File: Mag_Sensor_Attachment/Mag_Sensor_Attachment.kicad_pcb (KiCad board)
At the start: 2 copper layers, 14 x 15.8 mm, 5 parts, among them J2 Conn_01x06_Socket, U1 MA730

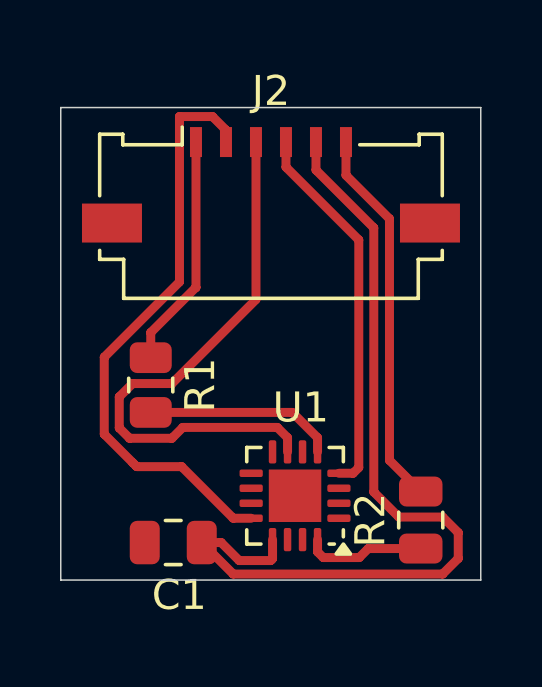
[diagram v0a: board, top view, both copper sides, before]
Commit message: Check up
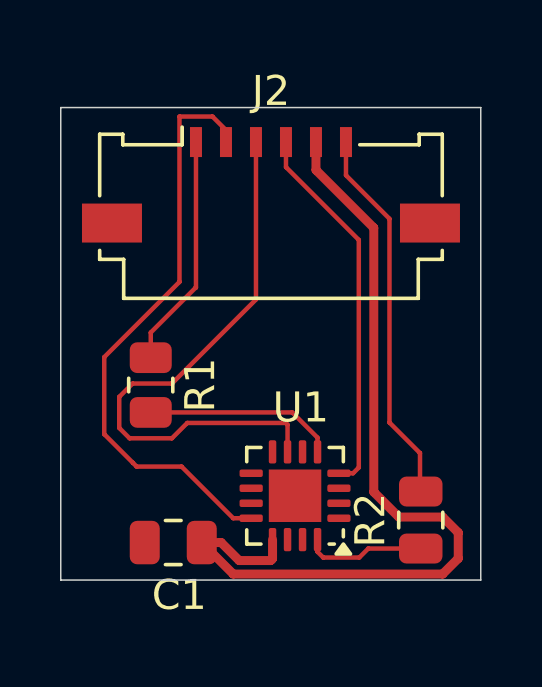
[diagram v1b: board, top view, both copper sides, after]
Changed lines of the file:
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@@
 		(start 152.434772 89.412272)
 		(end 150.0075 86.985)
-		(width 0.3)
+		(width 0.15)
 		(layer "F.Cu")
 		(net 3)
@@
 		(start 152.244772 97.19)
 		(end 152.434772 97)
-		(width 0.3)
+		(width 0.15)
 		(layer "F.Cu")
 		(net 3)
@@
 		(start 150.0075 86.985)
 		(end 150.0075 86.15)
-		(width 0.3)
+		(width 0.15)
 		(layer "F.Cu")
 		(net 3)
@@
 		(start 151.7725 97.19)
 		(end 152.244772 97.19)
-		(width 0.3)
+		(width 0.15)
 		(layer "F.Cu")
 		(net 3)
@@
 		(start 152.434772 97)
 		(end 152.434772 89.412272)
-		(width 0.3)
-		(layer "F.Cu")
-		(net 3)
-	)
-	(segment
-		(start 146.567956 95.6625)
+		(width 0.15)
+		(layer "F.Cu")
+		(net 3)
+	)
+	(segment
+		(start 144.894544 94.2)
+		(end 146.205456 94.2)
+		(width 0.15)
+		(layer "F.Cu")
+		(net 4)
+	)
+	(segment
+		(start 146.205456 96.025)
+		(end 144.794544 96.025)
+		(width 0.15)
+		(layer "F.Cu")
+		(net 4)
+	)
+	(segment
+		(start 150.06 96.4775)
+		(end 150.06 95.5725)
+		(width 0.15)
+		(layer "F.Cu")
+		(net 4)
+	)
+	(segment
+		(start 146.717956 95.5125)
 		(end 146.205456 96.025)
-		(width 0.3)
+		(width 0.15)
+		(layer "F.Cu")
+		(net 4)
+	)
+	(segment
+		(start 144.794544 96.025)
+		(end 144.45 95.680456)
+		(width 0.15)
 		(layer "F.Cu")
 		(net 4)
@@
 		(start 144.45 95.680456)
 		(end 144.45 94.644544)
-		(width 0.3)
-		(layer "F.Cu")
-		(net 4)
-	)
-	(segment
-		(start 146.205456 96.025)
-		(end 144.794544 96.025)
-		(width 0.3)
-		(layer "F.Cu")
-		(net 4)
-	)
-	(segment
-		(start 144.894544 94.2)
-		(end 146.205456 94.2)
-		(width 0.3)
+		(width 0.15)
+		(layer "F.Cu")
+		(net 4)
+	)
+	(segment
+		(start 150 95.5125)
+		(end 146.717956 95.5125)
+		(width 0.15)
+		(layer "F.Cu")
+		(net 4)
+	)
+	(segment
+		(start 149.0075 91.397956)
+		(end 149.0075 86.15)
+		(width 0.15)
+		(layer "F.Cu")
+		(net 4)
+	)
+	(segment
+		(start 144.45 94.644544)
+		(end 144.894544 94.2)
+		(width 0.15)
 		(layer "F.Cu")
 		(net 4)
@@
 		(start 146.205456 94.2)
 		(end 149.0075 91.397956)
-		(width 0.3)
-		(layer "F.Cu")
-		(net 4)
-	)
-	(segment
-		(start 149.717596 95.6625)
-		(end 146.567956 95.6625)
-		(width 0.3)
-		(layer "F.Cu")
-		(net 4)
-	)
-	(segment
-		(start 144.794544 96.025)
-		(end 144.45 95.680456)
-		(width 0.3)
-		(layer "F.Cu")
-		(net 4)
-	)
-	(segment
-		(start 149.0075 91.397956)
-		(end 149.0075 86.15)
-		(width 0.3)
-		(layer "F.Cu")
-		(net 4)
-	)
-	(segment
-		(start 150.06 96.4775)
-		(end 150.06 96.004904)
-		(width 0.3)
-		(layer "F.Cu")
-		(net 4)
-	)
-	(segment
-		(start 150.06 96.004904)
-		(end 149.717596 95.6625)
-		(width 0.3)
-		(layer "F.Cu")
-		(net 4)
-	)
-	(segment
-		(start 144.45 94.644544)
-		(end 144.894544 94.2)
-		(width 0.3)
+		(width 0.15)
+		(layer "F.Cu")
+		(net 4)
+	)
+	(segment
+		(start 150.06 95.5725)
+		(end 150 95.5125)
+		(width 0.15)
 		(layer "F.Cu")
 		(net 4)
@@
 		(start 147 91)
 		(end 147.0075 91)
-		(width 0.3)
+		(width 0.15)
 		(layer "F.Cu")
 		(net 5)
@@
 		(start 145.5 92.5)
 		(end 147 91)
-		(width 0.3)
+		(width 0.15)
 		(layer "F.Cu")
 		(net 5)
@@
 		(start 147.0075 91)
 		(end 147.0075 86.15)
-		(width 0.3)
+		(width 0.15)
 		(layer "F.Cu")
 		(net 5)
@@
 		(start 145.5 93.3375)
 		(end 145.5 92.5)
-		(width 0.3)
+		(width 0.15)
 		(layer "F.Cu")
 		(net 5)
@@
 		(start 146.4575 90.812044)
 		(end 146.4575 85.3)
-		(width 0.3)
+		(width 0.15)
 		(layer "F.Cu")
 		(net 6)
@@
 		(start 145.031218 96.968782)
 		(end 144.906218 96.843782)
-		(width 0.3)
+		(width 0.15)
 		(layer "F.Cu")
 		(net 6)
@@
 		(start 143.95 93.319544)
 		(end 146.4575 90.812044)
-		(width 0.3)
+		(width 0.15)
 		(layer "F.Cu")
 		(net 6)
@@
 		(start 148.25 98.69)
 		(end 146.528782 96.968782)
-		(width 0.3)
+		(width 0.15)
 		(layer "F.Cu")
 		(net 6)
@@
 		(start 144.906218 96.843782)
 		(end 143.95 95.887563)
-		(width 0.3)
+		(width 0.15)
 		(layer "F.Cu")
 		(net 6)
@@
 		(start 147.5575 85.3)
 		(end 148.0075 85.75)
-		(width 0.3)
+		(width 0.15)
 		(layer "F.Cu")
 		(net 6)
@@
 		(start 148.0075 85.75)
 		(end 148.0075 86.15)
-		(width 0.3)
+		(width 0.15)
 		(layer "F.Cu")
 		(net 6)
@@
 		(start 146.528782 96.968782)
 		(end 145.031218 96.968782)
-		(width 0.3)
+		(width 0.15)
 		(layer "F.Cu")
 		(net 6)
@@
 		(start 143.95 95.887563)
 		(end 143.95 93.319544)
-		(width 0.3)
+		(width 0.15)
 		(layer "F.Cu")
 		(net 6)
@@
 		(start 146.4575 85.3)
 		(end 147.5575 85.3)
-		(width 0.3)
+		(width 0.15)
 		(layer "F.Cu")
 		(net 6)
@@
 		(start 148.8475 98.69)
 		(end 148.25 98.69)
-		(width 0.3)
+		(width 0.15)
 		(layer "F.Cu")
 		(net 6)
@@
 		(start 152.0075 87.2575)
 		(end 152.0075 86.15)
-		(width 0.3)
+		(width 0.15)
 		(layer "F.Cu")
 		(net 7)
@@
 		(start 153.4575 88.7075)
 		(end 152.0075 87.2575)
-		(width 0.3)
-		(layer "F.Cu")
-		(net 7)
-	)
-	(segment
-		(start 153.4575 96.7575)
+		(width 0.15)
+		(layer "F.Cu")
+		(net 7)
+	)
+	(segment
+		(start 154.475 96.5175)
+		(end 153.4575 95.5)
+		(width 0.15)
+		(layer "F.Cu")
+		(net 7)
+	)
+	(segment
+		(start 154.475 97.775)
+		(end 154.475 96.5175)
+		(width 0.15)
+		(layer "F.Cu")
+		(net 7)
+	)
+	(segment
+		(start 153.4575 95.5)
 		(end 153.4575 88.7075)
-		(width 0.3)
+		(width 0.15)
 		(layer "F.Cu")
 		(net 7)
@@
 	(segment
 		(start 154.5 97.8)
-		(end 153.4575 96.7575)
-		(width 0.3)
+		(end 154.475 97.775)
+		(width 0.15)
 		(layer "F.Cu")
 		(net 7)
@@
 		(start 151.06 96.004904)
 		(end 151.06 96.4775)
-		(width 0.3)
+		(width 0.15)
 		(layer "F.Cu")
 		(net 8)
@@
 		(start 150.217596 95.1625)
 		(end 151.06 96.004904)
-		(width 0.3)
+		(width 0.15)
 		(layer "F.Cu")
 		(net 8)
@@
 		(start 145.5 95.1625)
 		(end 150.217596 95.1625)
-		(width 0.3)
+		(width 0.15)
 		(layer "F.Cu")
 		(net 8)
@@
 		(start 152.75 99.7)
 		(end 154.5 99.7)
-		(width 0.3)
+		(width 0.15)
 		(layer "F.Cu")
 		(net 9)
@@
 		(start 151.06 99.81)
 		(end 151.25 100)
-		(width 0.3)
+		(width 0.15)
 		(layer "F.Cu")
 		(net 9)
@@
 		(start 151.06 99.4025)
 		(end 151.06 99.81)
-		(width 0.3)
+		(width 0.15)
 		(layer "F.Cu")
 		(net 9)
@@
 		(start 151.25 100)
 		(end 152.45 100)
-		(width 0.3)
+		(width 0.15)
 		(layer "F.Cu")
 		(net 9)
@@
 		(start 152.45 100)
 		(end 152.75 99.7)
-		(width 0.3)
-		(layer "F.Cu")
-		(net 9)
+		(width 0.15)
+		(layer "F.Cu")
+		(net 9)
